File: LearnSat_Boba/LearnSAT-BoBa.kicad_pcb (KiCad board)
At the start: 4 copper layers, 90.3 x 95.8 mm, 71 parts, among them J1 DF13C-2P-1.25V(21), J2 DF13C-2P-1.25V(21), J3 DF13C-2P-1.25V(21), J4 DF13C-2P-1.25V(21), Q1 FQD13N06LTM, Q2 FQD13N06LTM, U1 LTC4231HUD-2#TRPBF, U2 INA219, U3 INA219AIDCNR, U4_IN-A LTC4231IUD-2#TRPBF, U4_IN-B LTC4231IUD-2#TRPBF, U4_IN-C LTC4231IUD-2#TRPBF, U4_IN-E LTC4231IUD-2#TRPBF, U4_IN-F LTC4231IUD-2#TRPBF, U4_IN-G LTC4231IUD-2#TRPBF, U5 INA219AIDCNR

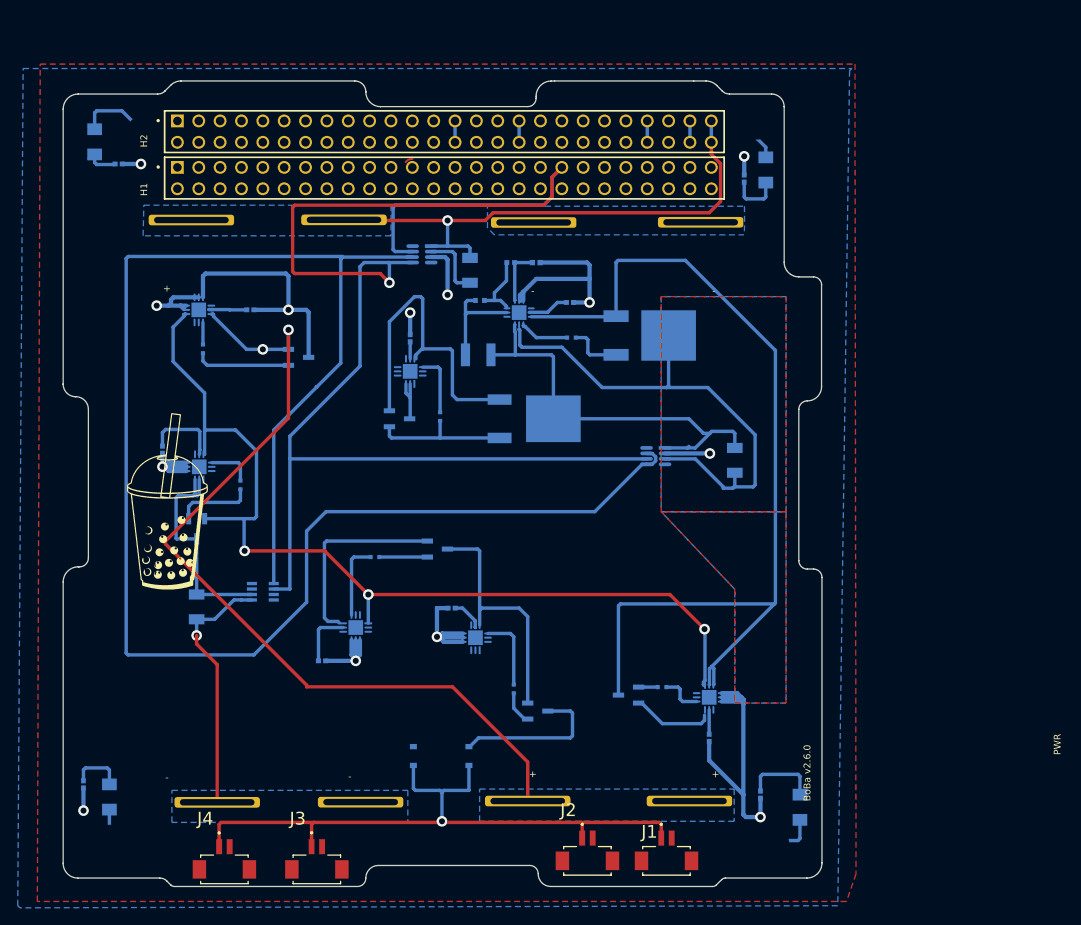
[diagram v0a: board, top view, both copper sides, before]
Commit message: Update LearnSAT-BoBa.kicad_pcb
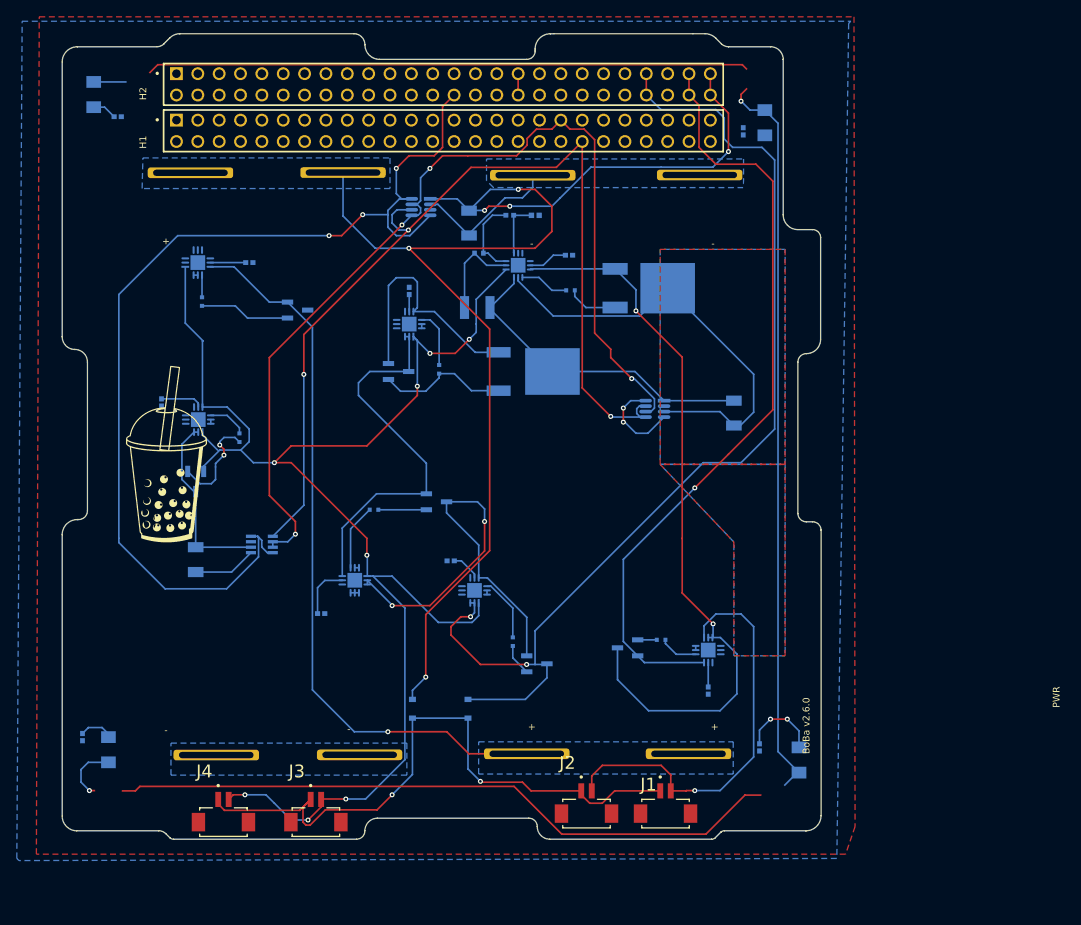
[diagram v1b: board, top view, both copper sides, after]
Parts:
- removed the ? at (188.1, 147.7)
- removed the ? at (136.8, 73.6)
- removed the ? at (179.2, 73.9)
- removed the ? at (108.9, 147.2)
- removed the ? at (106.6, 135.0)
- removed the ? at (177.9, 142.7)
- removed the ? at (112.6, 62.9)
- removed the ? at (118.6, 73.6)
- removed the ? at (106.6, 75.6)
- removed the ? at (186.0, 75.4)
- removed the ? at (158.6, 142.7)
- removed the ? at (138.8, 142.9)
- removed the ? at (190.5, 135.0)
- removed the ? at (159.3, 73.9)
- removed the ? at (186.0, 62.5)
- removed the ? at (121.7, 142.9)
- added ?: , , F.Cu at (185.8, 69.8)
- added ?: , , F.Cu at (106.4, 70.0)
- added ?: , , F.Cu at (177.7, 137.1)
- added ?: , , F.Cu at (188.0, 142.0)
- added ?: , , F.Cu at (118.5, 68.0)
- added ?: , , F.Cu at (158.5, 137.1)
- added ?: , , F.Cu at (190.3, 129.3)
- added ?: , , F.Cu at (112.5, 57.3)
- added ?: , , F.Cu at (121.6, 137.3)
- added ?: , , F.Cu at (185.8, 56.9)
- added ?: , , F.Cu at (136.7, 68.0)
- added ?: , , F.Cu at (138.6, 137.2)
- added ?: , , F.Cu at (106.4, 129.3)
- added ?: , , F.Cu at (108.8, 141.5)
- added ?: , , F.Cu at (179.1, 68.3)
- added ?: , , F.Cu at (159.2, 68.3)
- moved 1_IN-F 5.62 mm to (119.1, 104.7)
- moved 1_IN-G 5.62 mm to (131.3, 84.4)
- moved C4_IN-B 5.62 mm to (134.1, 120.4)
- moved C4_IN-C 5.62 mm to (144.5, 82.1)
- moved C4_IN-E 5.62 mm to (180.1, 129.6)
- moved C4_IN-F 5.62 mm to (115.1, 95.3)
- moved C4_IN-G 5.62 mm to (125.5, 78.7)
- moved D1 5.62 mm to (151.5, 131.8)
- moved D2 5.62 mm to (144.9, 131.8)
- moved FB2 5.62 mm to (184.3, 63.1)
- moved FB3 5.62 mm to (105.7, 135.1)
- moved J3 5.62 mm to (133.4, 145.2)
- moved J4 5.62 mm to (122.4, 145.2)
- moved R1 5.62 mm to (152.6, 84.0)
- moved R10 5.62 mm to (108.8, 136.6)
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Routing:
- net Chassis GND: track 22.0 -> 264.1 mm, vias 0 -> 2
- net GND: track 151.9 -> 1.00 mm, vias 13 -> 0
- net 3V3_Secondary: track 2.54 -> 133.4 mm, vias 0 -> 5
- net INHIBIT: track 113.0 -> 221.8 mm, vias 3 -> 9
- net Vmppt: track 21.1 -> 128.1 mm, vias 0 -> 2
- net Pack+_Pos: track 64.7 -> 157.7 mm, vias 1 -> 6
- net I2C Clock: track 204.3 -> 115.3 mm, vias 0 -> 3
- net VBatt: track 12.1 -> 92.5 mm, vias 0 -> 1
- net I2C Data: track 181.0 -> 117.5 mm, vias 1 -> 4
- net D_IN-E: track 114.6 -> 88.1 mm, vias 0 -> 2
- net Pack+_Neg: track 30.3 -> 7.53 mm, vias 1 -> 0
- net D_IN-B: track 29.2 -> 51.2 mm, vias 0 -> 2
- net Pack-_Pos: track 103.4 -> 86.9 mm, vias 2 -> 1
- net D_IN-C: track 29.2 -> 45.1 mm
- net NetQ1_4: track 49.1 -> 38.5 mm
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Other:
- board size 90.3 x 95.8 mm -> 90.2 x 95.8 mm
